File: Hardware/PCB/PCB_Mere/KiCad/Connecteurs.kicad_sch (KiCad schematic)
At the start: 12 parts, among them CN2 B4B-PH-K-S_GNSS, U5 B8B-PH-K-S-_TACTIL, U6 B8B-PH-K-S_FILS, U7 B10B-PH-K-S-_SCRN/JOY/ALIM

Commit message: last version
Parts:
- C31, C32, C36, C37, C38, C39: LCSC Part C49062 -> C1525
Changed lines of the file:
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@@
 			)
 		)
-		(property "LCSC Part" "C49062"
+		(property "LCSC Part" "C1525"
 			(at 242.57 30.48 90)
 			(hide yes)
@@
 			)
 		)
-		(property "LCSC Part" "C49062"
+		(property "LCSC Part" "C1525"
 			(at 52.07 86.36 0)
 			(hide yes)
@@
 			)
 		)
-		(property "LCSC Part" "C49062"
+		(property "LCSC Part" "C1525"
 			(at 228.6 31.75 90)
 			(hide yes)
@@
 			)
 		)
-		(property "LCSC Part" "C49062"
+		(property "LCSC Part" "C1525"
 			(at 48.26 88.9 0)
 			(hide yes)
@@
 			)
 		)
-		(property "LCSC Part" "C49062"
+		(property "LCSC Part" "C1525"
 			(at 168.91 105.41 0)
 			(hide yes)
@@
 			)
 		)
-		(property "LCSC Part" "C49062"
+		(property "LCSC Part" "C1525"
 			(at 38.1 153.67 0)
 			(hide yes)

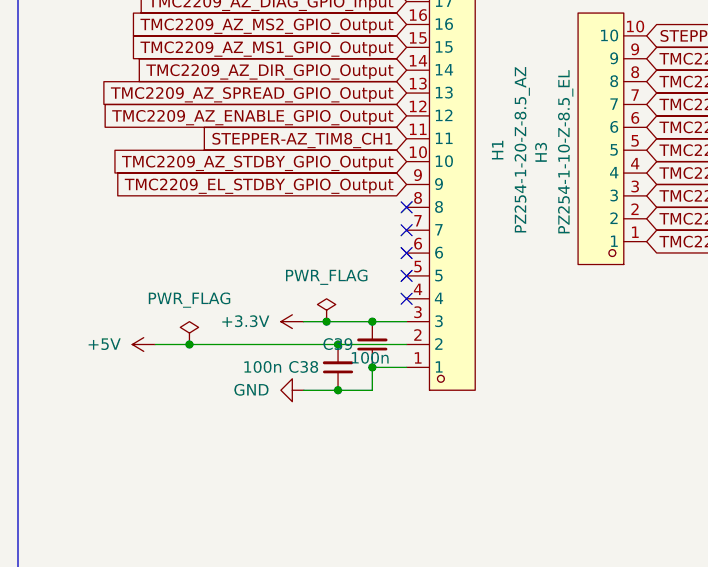
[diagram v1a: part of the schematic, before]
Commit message: last version
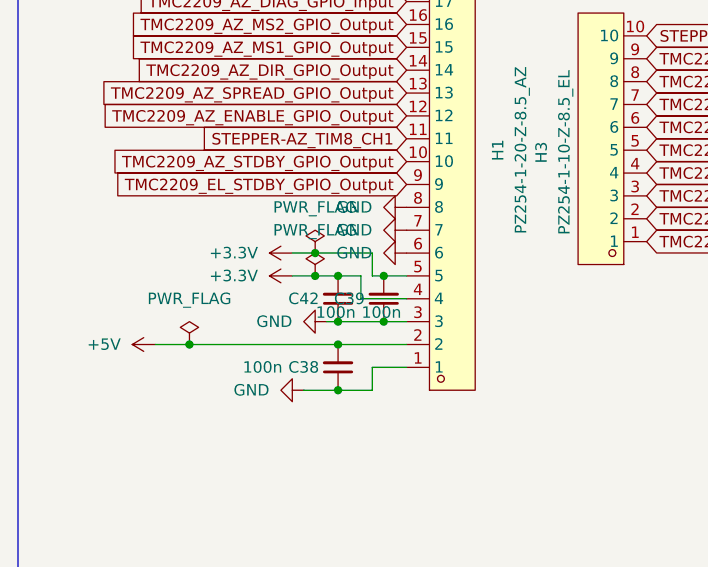
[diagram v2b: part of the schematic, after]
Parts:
- added C42: 100n, Capacitor_SMD:C_0402_1005Metric, symbol Device:C_Small
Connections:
- net +3.3V: now also H1.4, H1.5, C42.2; no longer H1.3
- net GND: now also H1.3, H1.6, H1.7, H1.8, C42.1
- no-connect marks 5 -> 0
